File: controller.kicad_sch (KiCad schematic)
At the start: 26 parts, among them J5 Conn_01x10_Pin, J6 Conn_01x10_Pin, J8 AVR-ISP-6, Q1 BSS138, Q2 BSS138, Q3 BSS138, U10 ATmega328PB-A, Y1 16M

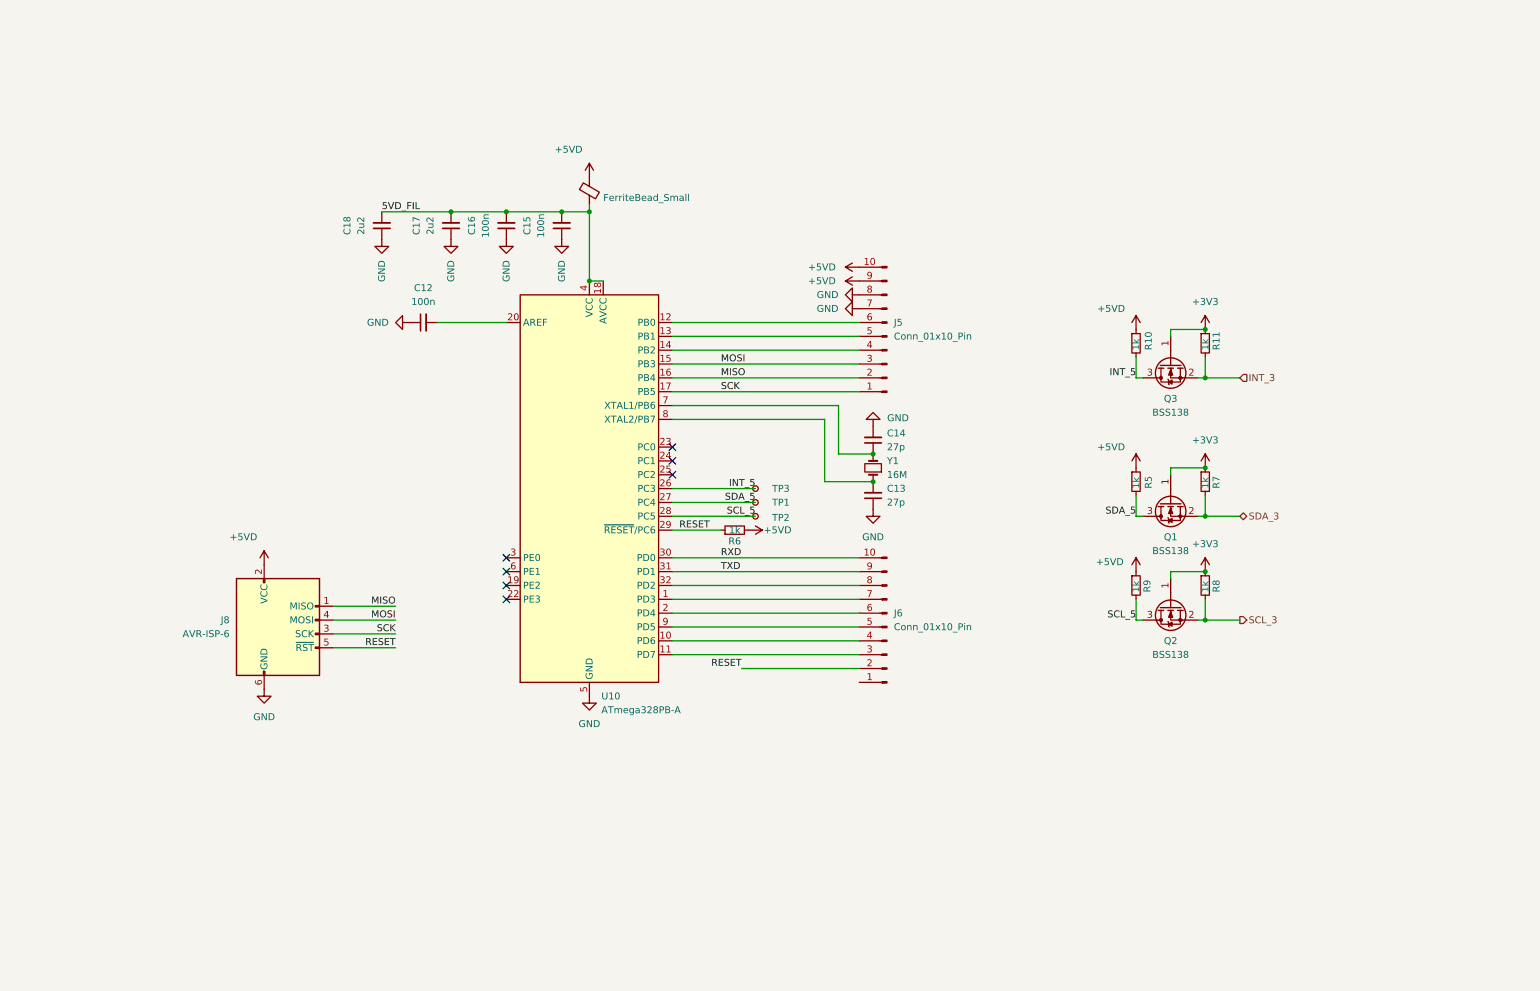
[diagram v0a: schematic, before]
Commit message: weiter layoutet...
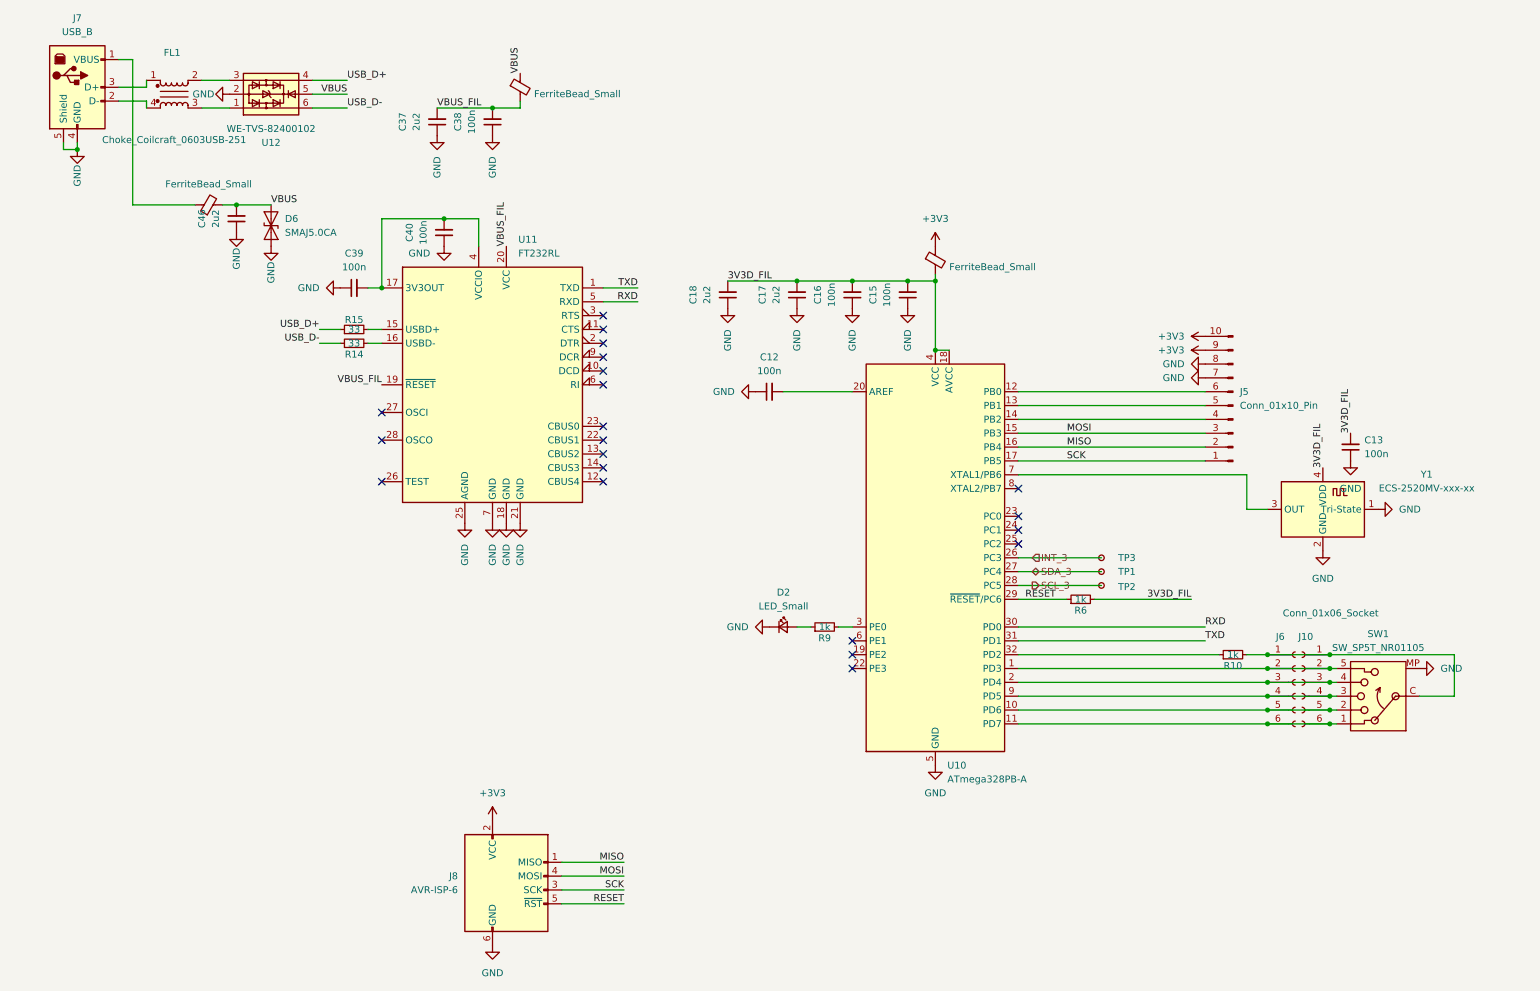
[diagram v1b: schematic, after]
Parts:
- removed C14: 27p, symbol Device:C_Small
- removed J6: Conn_01x10_Pin, symbol Connector:Conn_01x10_Pin
- removed Q1, Q2, Q3: BSS138, Package_TO_SOT_SMD:SOT-23, symbol Transistor_FET:BSS138
- removed R11, R5, R7, R8: 1k, symbol Device:R_Small
- removed Y1: 16M, Crystal:Crystal_SMD_HC49-SD, symbol Device:Crystal_Small
- added C37, C46: 2u2, Capacitor_SMD:C_0805_2012Metric_Pad1.18x1.45mm_HandSolder, symbol Device:C_Small
- added C38, C39, C40: 100n, Capacitor_SMD:C_0805_2012Metric_Pad1.18x1.45mm_HandSolder, symbol Device:C_Small
- added D2: LED_Small, LED_SMD:LED_0805_2012Metric_Pad1.15x1.40mm_HandSolder, symbol Device:LED_Small
- added D6: SMAJ5.0CA, Diode_SMD:D_SMA, symbol Diode:SMAJ5.0CA
- added FB5, FB6: FerriteBead_Small, Inductor_SMD:L_0805_2012Metric_Pad1.15x1.40mm_HandSolder, symbol Device:FerriteBead_Small
- added FL1: Choke_Coilcraft_0603USB-251, Inductor_SMD:L_CommonModeChoke_Coilcraft_0603USB, symbol Filter:Choke_Coilcraft_0603USB-251
- added J10: Conn_01x06_Socket, Connector_PinHeader_2.54mm:PinHeader_1x06_P2.54mm_Vertical, symbol Connector:Conn_01x06_Socket
- added J6: Conn_01x06_Socket, Connector_PinHeader_2.54mm:PinHeader_1x06_P2.54mm_Horizontal, symbol Connector:Conn_01x06_Socket
- added J7: USB_B, Connector_USB:USB_B_Lumberg_2411_02_Horizontal, symbol Connector:USB_B
- added R14, R15: 33, Resistor_SMD:R_0805_2012Metric_Pad1.20x1.40mm_HandSolder, symbol Device:R_Small
- added SW1: SW_SP5T_NR01105, Button_Switch_THT:SW_NKK_NR01, symbol Switch:SW_SP5T_NR01105
- added U11: FT232RL, Package_SO:SSOP-28_5.3x10.2mm_P0.65mm, symbol Interface_USB:FT232RL
- added U12: WE-TVS-82400102, Package_TO_SOT_SMD:SOT-23-6, symbol Power_Protection:WE-TVS-82400102
- added Y1: ECS-2520MV-xxx-xx, Oscillator:Oscillator_SMD_ECS_2520MV-xxx-xx-4Pin_2.5x2.0mm, symbol Oscillator:ECS-2520MV-xxx-xx
- C12, C15, C16, C17, C18: footprint (none) -> Capacitor_SMD:C_0805_2012Metric_Pad1.18x1.45mm_HandSolder
- C13: value 27p -> 100n; footprint (none) -> Capacitor_SMD:C_0805_2012Metric_Pad1.18x1.45mm_HandSolder
- FB3: footprint Inductor_SMD:L_0805_2012Metric_Pad1.05x1.20mm_HandSolder -> Inductor_SMD:L_0805_2012Metric_Pad1.15x1.40mm_HandSolder
- J5: footprint (none) -> Connector_PinHeader_2.54mm:PinHeader_1x10_P2.54mm_Vertical
- J8: footprint Connector_IDC:IDC-Header_2x05_P2.54mm_Vertical -> Connector_IDC:IDC-Header_2x03_P2.54mm_Vertical
- R10, R6, R9: footprint (none) -> Resistor_SMD:R_0805_2012Metric_Pad1.20x1.40mm_HandSolder
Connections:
- net SDA_5 is gone; now on net SDA_3: TP1.1, U10.27 (PC4)
- net +3V3: now also FB3.1, J5.10 (Pin_10), J5.9 (Pin_9), J8.2 (VCC)
- net GND: now also C37.1, C38.1, C39.1, C40.1, C46.1, D2.1 (K), D6.1 (A1), J7.4 (GND), J7.5 (Shield), SW1.MP, U11.18 (GND), U11.21 (GND), U11.25 (AGND), U11.7 (GND), U12.2, Y1.1 (Tri-State), Y1.2 (GND)
- net INT_3: now also TP3.1, U10.26 (PC3)
- net RXD: now also U11.5 (RXD)
- net SCL_3: now also TP2.1, U10.28 (PC5)
- net TXD: now also U11.1 (TXD)
- net at U10.8 (XTAL2/PB7): no longer C13.2
- net at U10.1 (PD3): now also J10.2 (Pin_2), J6.2 (Pin_2), SW1.5
- net at U10.10 (PD6): now also J10.5 (Pin_5), J6.5 (Pin_5), SW1.2
- net at U10.11 (PD7): now also J10.6 (Pin_6), J6.6 (Pin_6), SW1.1
- net at U10.2 (PD4): now also J10.3 (Pin_3), J6.3 (Pin_3), SW1.4
- net at U10.3 (PE0): now also R9.2
- net at U10.32 (PD2): now also R10.1
- net at U10.7 (XTAL1/PB6): now also Y1.3 (OUT)
- net at U10.9 (PD5): now also J10.4 (Pin_4), J6.4 (Pin_4), SW1.3
- removed net +5VD: FB3.1, J5.10 (Pin_10), J5.9 (Pin_9), J8.2 (VCC), R10.1, R6.2, R9.1
- net 5VD_FIL renamed 3V3D_FIL
- net 3V3D_FIL: now also C13.2, R6.2, Y1.4 (VDD)
- removed net INT_5: R10.2, TP3.1, U10.26 (PC3)
- removed net SCL_5: R9.2, TP2.1, U10.28 (PC5)
- new net: FB6.1, J7.1 (VBUS)
- new net: FL1.4, J7.2 (D-)
- new net: FL1.1, J7.3 (D+)
- new net: FL1.3, U12.1
- new net: FL1.2, U12.3
- new net: J10.1 (Pin_1), J6.1 (Pin_1), R10.2, SW1.C (Common)
- new net: R15.2, U11.15 (USBD+)
- new net: R14.2, U11.16 (USBD-)
- new net: C39.2, C40.2, U11.17 (3V3OUT), U11.4 (VCCIO)
- new net: D2.2 (A), R9.1
- new net USB_D+: R15.1, U12.4
- new net USB_D-: R14.1, U12.6
- new net VBUS: C46.2, D6.2 (A2), FB5.1, FB6.2, U12.5
- new net VBUS_FIL: C37.2, C38.2, FB5.2, U11.19 (~{RESET}), U11.20 (VCC)
- no-connect marks 7 -> 21
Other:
- moved on the sheet: C12, C15, C16, C17, C18, J5, J8, R6, TP1, TP2, TP3, U10

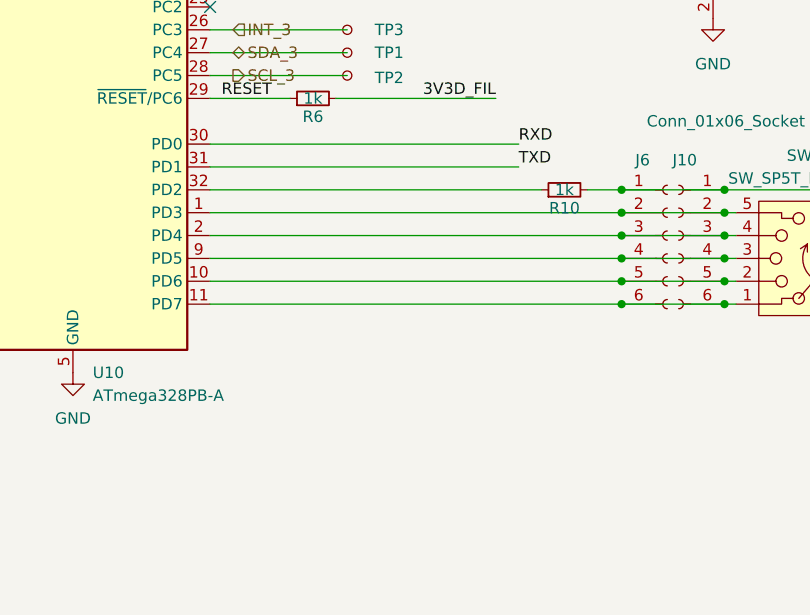
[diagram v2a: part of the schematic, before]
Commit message: noch ein paar Kleinigkeiten
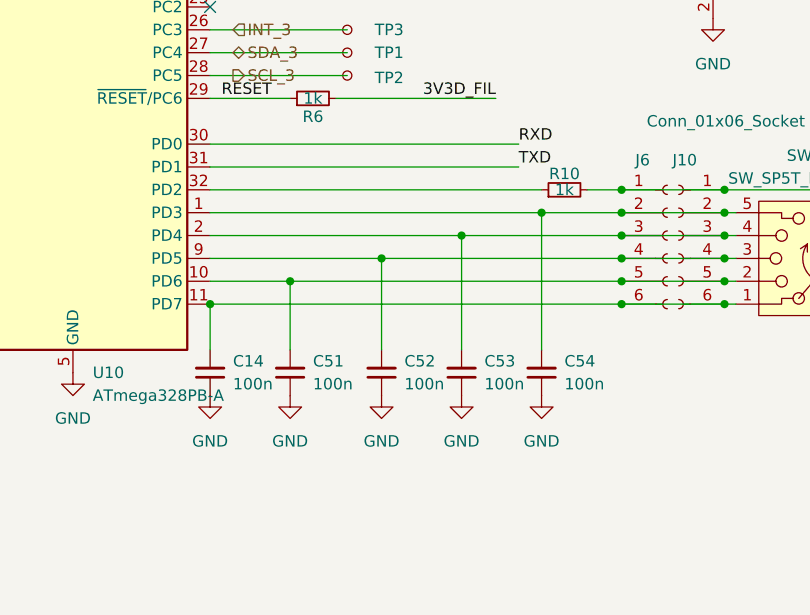
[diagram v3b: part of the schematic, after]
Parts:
- added C14, C51, C52, C53, C54: 100n, Capacitor_SMD:C_0805_2012Metric_Pad1.18x1.45mm_HandSolder, symbol Device:C_Small
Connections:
- net GND: now also C14.1, C51.1, C52.1, C53.1, C54.1
- net at J10.2 (Pin_2), J6.2 (Pin_2), SW1.5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: now also C54.2
- net at J10.5 (Pin_5), J6.5 (Pin_5), SW1.2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: now also C51.2
- net at J10.6 (Pin_6), J6.6 (Pin_6), SW1.1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: now also C14.2
- net at J10.3 (Pin_3), J6.3 (Pin_3), SW1.4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: now also C53.2
- net at J10.4 (Pin_4), J6.4 (Pin_4), SW1.3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: now also C52.2

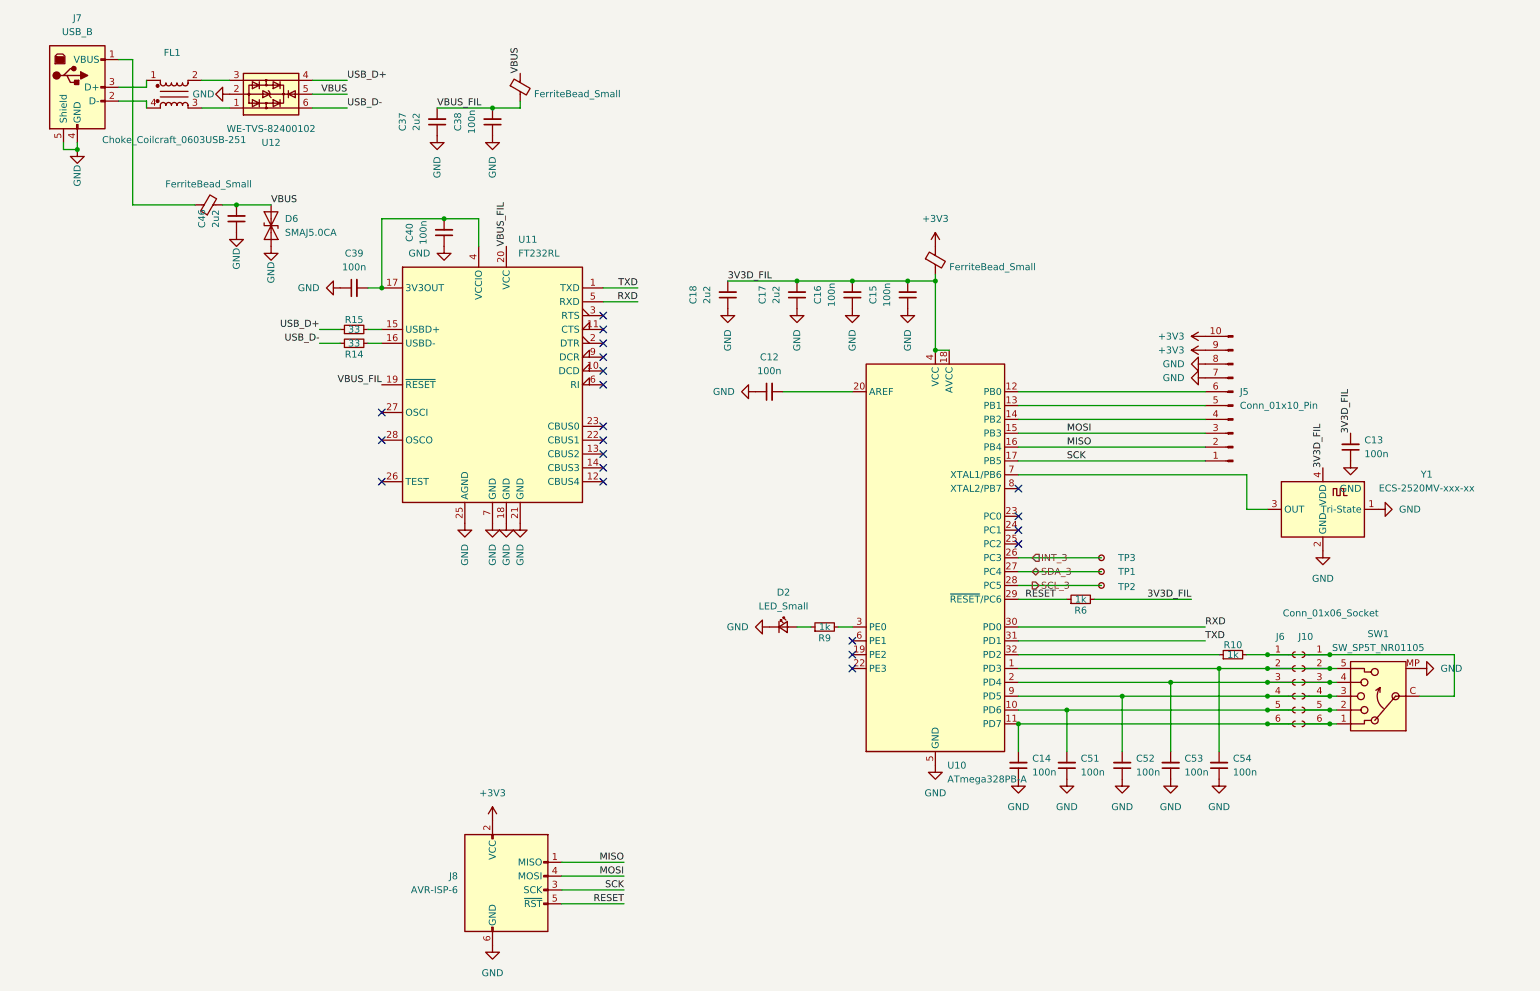
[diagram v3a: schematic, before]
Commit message: BOM angefangen und im Layout vom Hundertsten ins Tausendste gekommen...
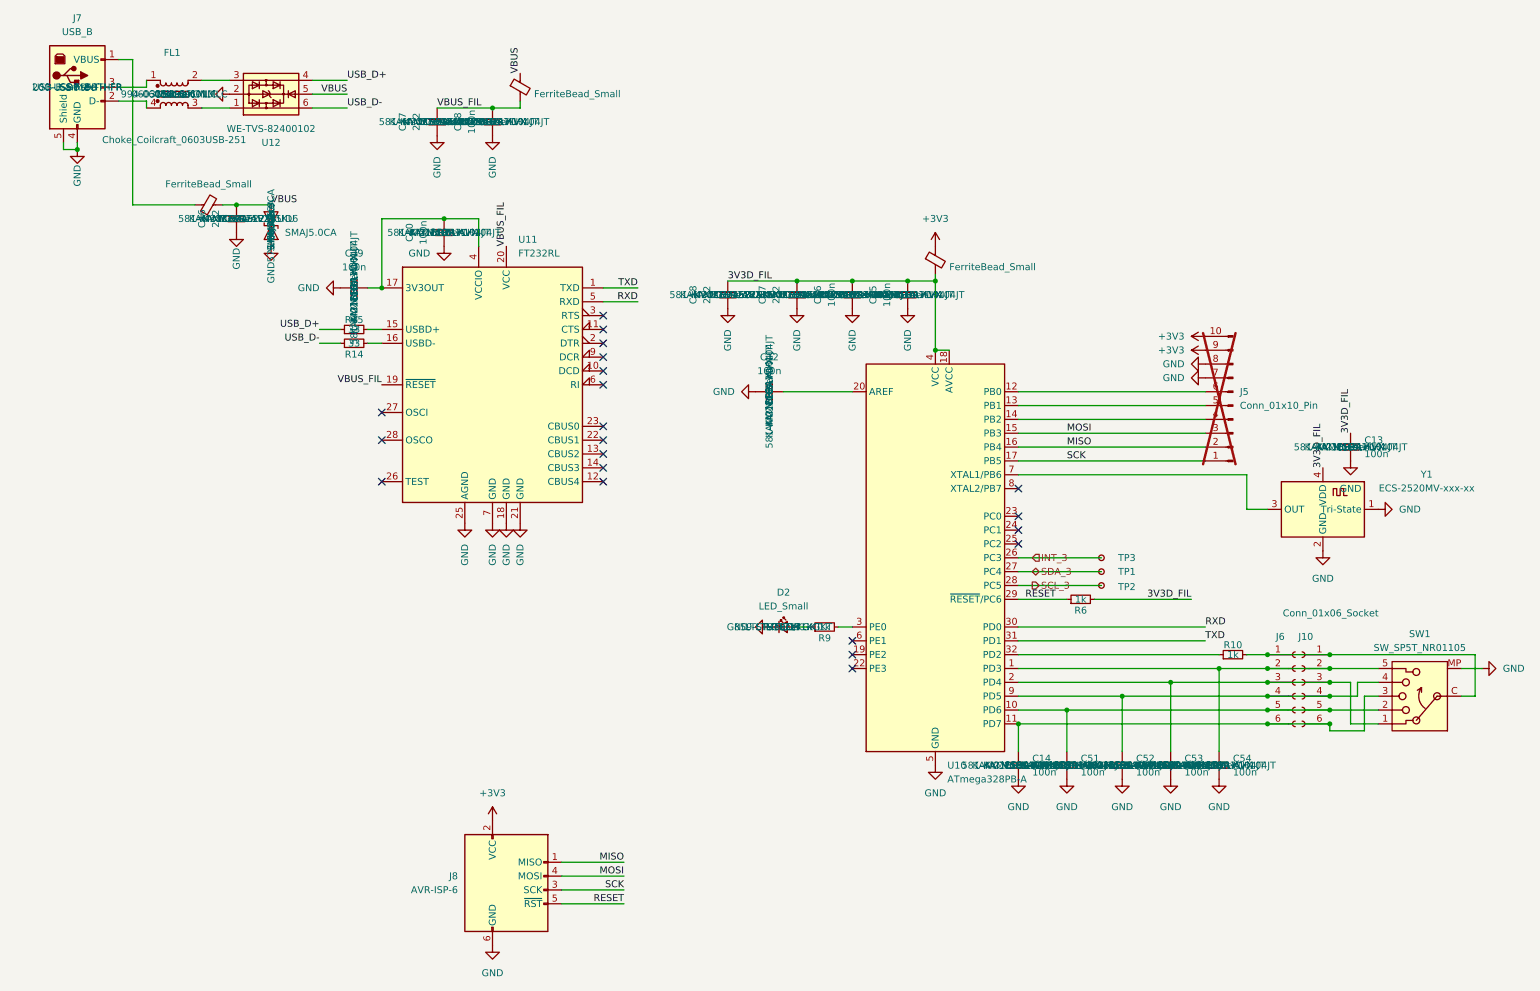
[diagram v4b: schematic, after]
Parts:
- C12, C13, C14, C15, C16, C38, C39, C40, C51, C52, C53, C54: Distributor (none) -> Mouser; Distributor PN (none) -> 581-KAM21BR71H104JT; Manufacturer (none) -> KYOCERA AVX; Manufacturer PN (none) -> KAM21BR71H104JT
- C17, C18, C37, C46: Distributor (none) -> Mouser; Distributor PN (none) -> 581-KAM21KR71E225KU; Manufacturer (none) -> KYOCERA AVX; Manufacturer PN (none) -> KAM21KR71E225KU
- D2: Distributor (none) -> Mouser; Distributor PN (none) -> 859-LTST-C171KGKT; Manufacturer (none) -> LITEON; Manufacturer PN (none) -> LTST-C171KGKT
- D6: Distributor (none) -> Mouser; Distributor PN (none) -> 576-SMAJ5.0CA; Manufacturer (none) -> Littelfuse; Manufacturer PN (none) -> SMAJ5.0CA
- FL1: Distributor (none) -> Mouser; Distributor PN (none) -> 994-0603USB-601MLC; Manufacturer (none) -> Coilcraft; Manufacturer PN (none) -> 0603USB-601MLC
- J5: now not fitted
- J7: Distributor PN (none) -> 200-USBBSFBTHFR; Manufacturer (none) -> Samtec; Manufacturer PN (none) -> USB-B-S-F-B-TH-FR
- J8: Distributor (none) -> Mouser; Distributor PN (none) -> 737-BHR-06-VUA; Manufacturer (none) -> Adam Tech; Manufacturer PN (none) -> BHR-06-VUA
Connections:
- net at C53.2, J10.3 (Pin_3), J6.3 (Pin_3)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: now also SW1.1; no longer SW1.4
- net at C14.2, J10.6 (Pin_6), J6.6 (Pin_6)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: now also SW1.3; no longer SW1.1
- net at C52.2, J10.4 (Pin_4), J6.4 (Pin_4)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: now also SW1.4; no longer SW1.3
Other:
- moved on the sheet: SW1
